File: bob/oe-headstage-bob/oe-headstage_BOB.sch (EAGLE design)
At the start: 13 parts, among them U1 SN65LVDS1DBVR, U2 SN65LVDS2DBVR, U3 SN65LVDS1DBVR, U4 SN65LVDS1DBVR

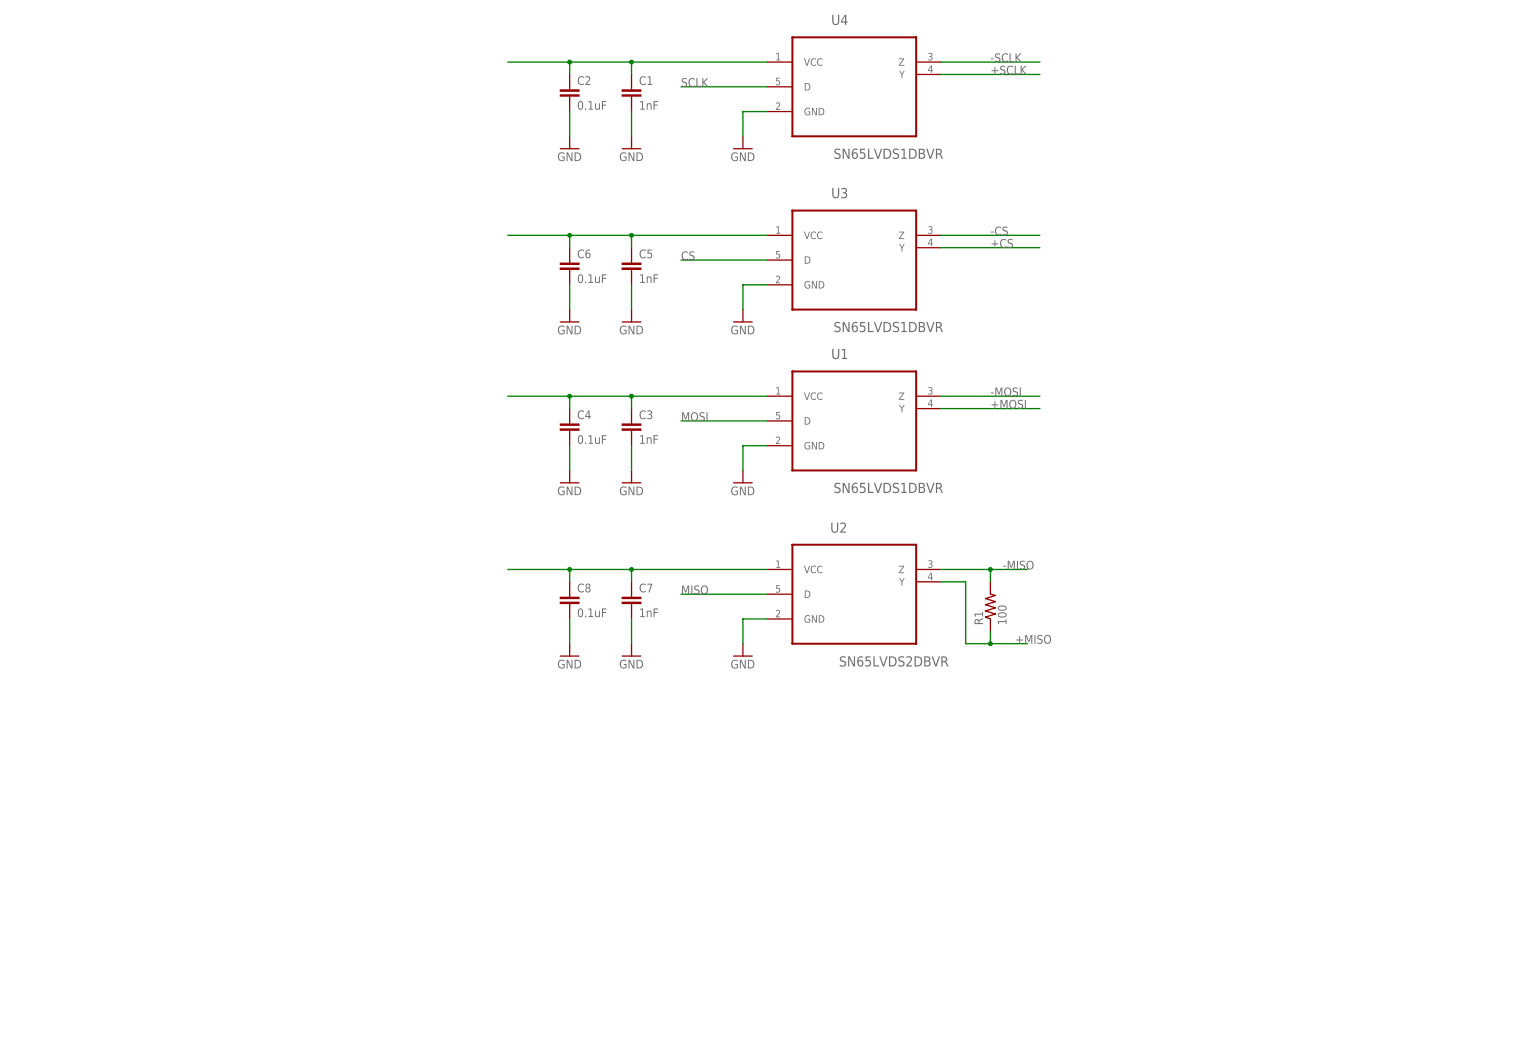
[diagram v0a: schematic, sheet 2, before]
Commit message: Minor.
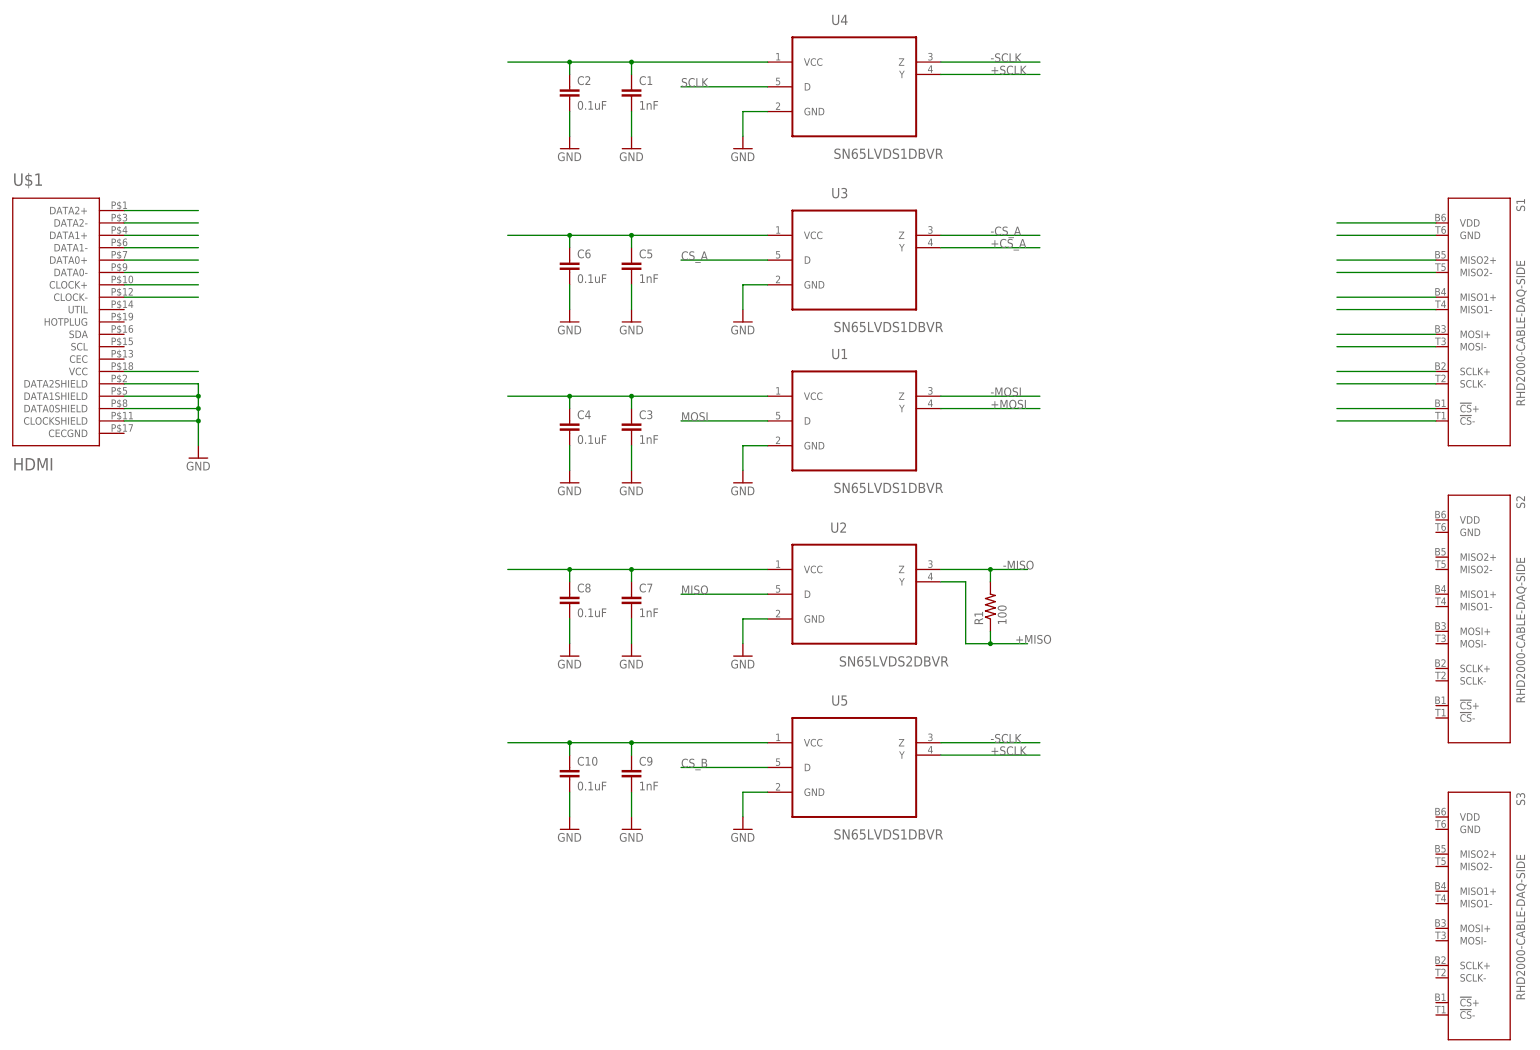
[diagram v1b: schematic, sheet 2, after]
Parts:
- added C10: 0.1uF, rcl:C-EUC0603
- added C9: 1nF, rcl:C-EUC0603
- added S1, S2, S3: RHD2000-CABLE-DAQ-SIDE, RHD2000_eval_board:RHD2000-CABLE-DAQ-SIDE
- added U$1: HDMI, open-ephys:HDMI
- added U5: SN65LVDS1DBVR, ti-extended:SN65LVDS1DBVR
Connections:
- net +CS renamed +CS_A
- net -CS renamed -CS_A
- net CS renamed CS_A
- new net CS_B: U5.D
- new net N$10: S1.MISO1-
- new net N$11: S1.MOSI+
- new net N$12: S1.MOSI-
- new net N$13: S1.SCLK+
- new net N$14: S1.SCLK-
- new net N$15: S1.!CS!+
- new net N$16: S1.!CS!-
- new net N$17: U$1.DATA1-
- new net N$18: U$1.DATA0+
- new net N$19: U$1.DATA0-
- new net N$20: U$1.CLOCK+
- new net N$21: U$1.CLOCK-
- new net N$5: C10.1, C9.1, U5.VCC
- new net N$6: S1.MISO2+
- new net N$7: U$1.DATA1+
- new net N$8: S1.MISO2-
- new net N$9: S1.MISO1+
- new net VDRIVE: C1.1, C2.1, C5.1, C6.1, S1.VDD, U$1.VCC, U3.VCC, U4.VCC
- net +SCLK: now also U5.Y
- net -SCLK: now also U5.Z
- net GND: now also C10.2, C9.2, S1.GND, U$1.CLOCKSHIELD, U$1.DATA0SHIELD, U$1.DATA1SHIELD, U$1.DATA2SHIELD, U5.GND
- net N$1: now also U$1.DATA2+; no longer C1.1, C2.1, U4.VCC
- net N$3: now also U$1.DATA2-; no longer C5.1, C6.1, U3.VCC
